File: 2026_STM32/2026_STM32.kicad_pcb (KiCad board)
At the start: 2 copper layers, 22 parts, among them J1 USB_B, J2 Conn_01x05_Pin, SW1 1825910-6, U1 SPX3819M5-L-3-3, U2 STM32C011F4P6, U3 KTD2026

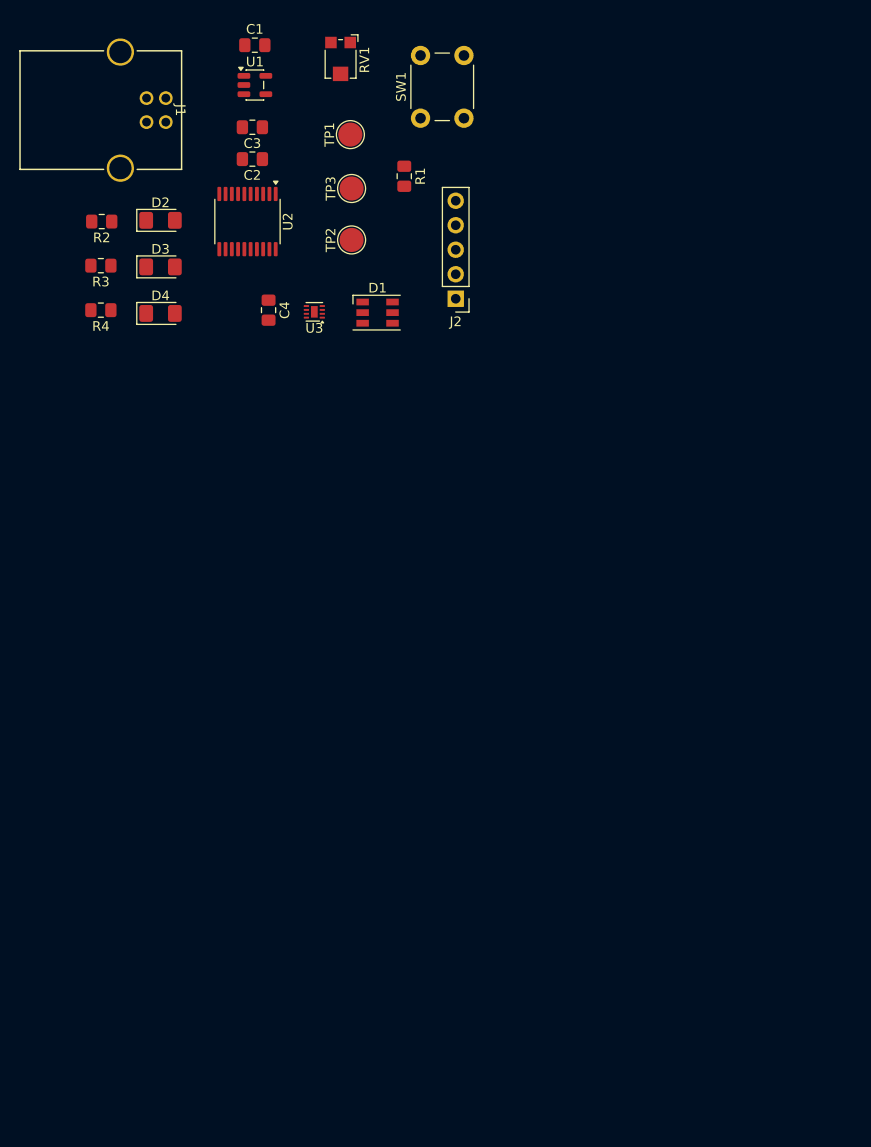
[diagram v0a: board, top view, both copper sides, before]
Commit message: stuff
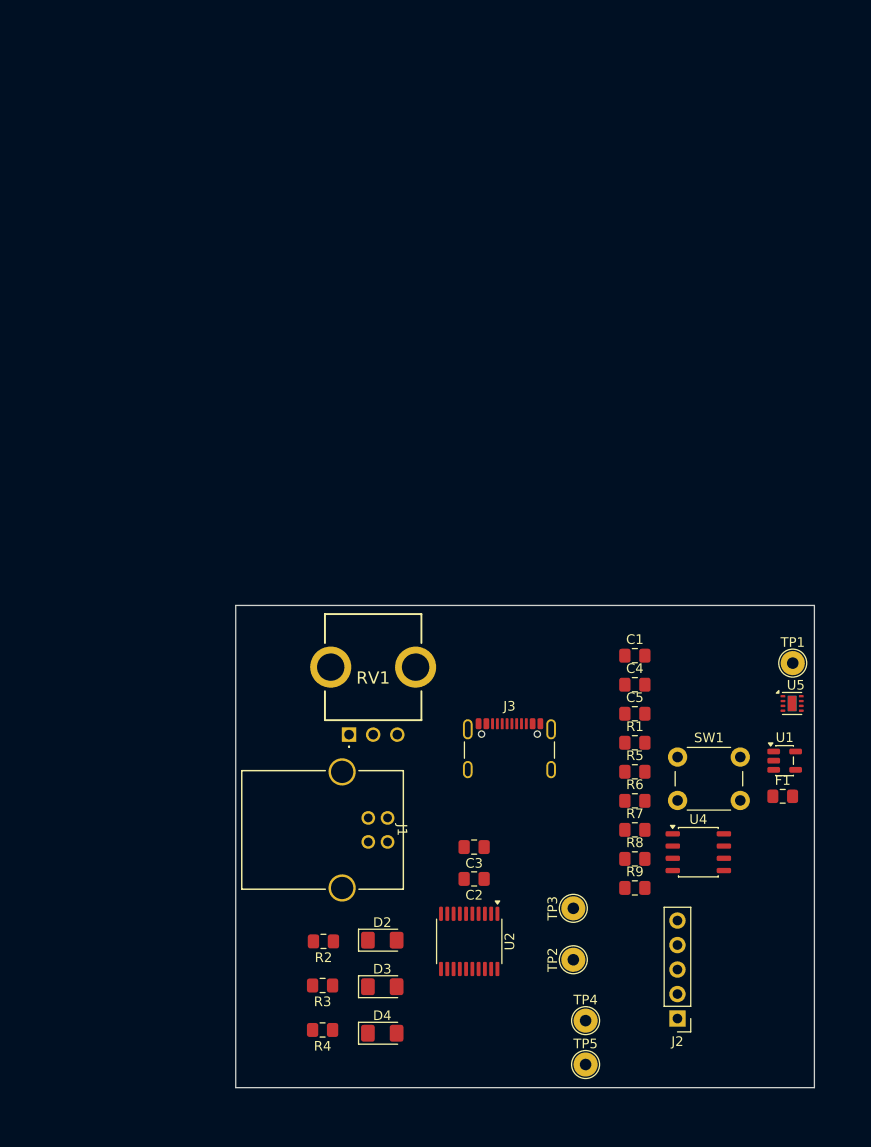
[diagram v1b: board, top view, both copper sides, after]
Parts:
- removed D1: CLX6F-FKC, LED_SMD:LED_RGB_PLCC-6
- removed U3: KTD2026, Package_DFN_QFN:DFN-8-1EP_1.5x1.5mm_P0.4mm_EP0.7x1.2mm
- added C5: 100nF, Capacitor_SMD:C_0805_2012Metric_Pad1.18x1.45mm_HandSolder, F.Cu at (141.4, 111.2)
- added F1: 0.5A, Fuse:Fuse_0805_2012Metric_Pad1.15x1.40mm_HandSolder, F.Cu at (156.7, 119.8)
- added J3: USB_C_Receptacle_USB2.0_16P, Connector_USB:USB_C_Receptacle_GCT_USB4105-xx-A_16P_TopMnt_Horizontal, F.Cu at (128.4, 115.9)
- added R5: 10kR, Capacitor_SMD:C_0805_2012Metric_Pad1.18x1.45mm_HandSolder, F.Cu at (141.4, 117.2)
- added R6: 10kR, Capacitor_SMD:C_0805_2012Metric_Pad1.18x1.45mm_HandSolder, F.Cu at (141.4, 120.3)
- added R7: 10kR, Capacitor_SMD:C_0805_2012Metric_Pad1.18x1.45mm_HandSolder, F.Cu at (141.4, 123.3)
- added R8: 5.1kR, Capacitor_SMD:C_0805_2012Metric_Pad1.18x1.45mm_HandSolder, F.Cu at (141.4, 126.3)
- added R9: 5.1kR, Capacitor_SMD:C_0805_2012Metric_Pad1.18x1.45mm_HandSolder, F.Cu at (141.4, 129.3)
- added TP4: TX, TestPoint:TestPoint_THTPad_D2.5mm_Drill1.2mm, F.Cu at (136.3, 143.1)
- added TP5: RX, TestPoint:TestPoint_THTPad_D2.5mm_Drill1.2mm, F.Cu at (136.3, 147.6)
- added U4: CH340N, Package_SO:JEITA_SOIC-8_3.9x4.9mm_P1.27mm, F.Cu at (148.0, 125.6)
- added U5: TMP1075DSG, Package_SON:WSON-8-1EP_2x2mm_P0.5mm_EP0.9x1.6mm_ThermalVias, F.Cu at (157.7, 110.2)
- C1: value 1.0uF -> 4.7uF
- C4: value 1.0uF -> 100nF
- R2: value 100R -> 330R
- RV1: footprint Potentiometer_SMD:Potentiometer_Bourns_TC33X_Vertical -> 2026 tutorial:PTV09A4015UB103
- TP1, TP2, TP3: footprint TestPoint:TestPoint_Pad_D2.5mm -> TestPoint:TestPoint_THTPad_D2.5mm_Drill1.2mm
- moved U1 89.0 mm to (156.9, 116.1)
- moved C3 78.1 mm to (124.7, 125.1)
- moved D4 78.1 mm to (115.2, 144.4)
- moved J1 78.1 mm to (115.7, 124.5)
- moved J2 78.1 mm to (145.8, 142.8)
- moved R3 78.1 mm to (109.0, 139.4)
- moved C2 78.1 mm to (124.7, 128.4)
- moved D2 78.1 mm to (115.2, 134.7)
- moved R2 78.1 mm to (109.1, 134.8)
- moved R4 78.1 mm to (109.0, 144.0)
- moved TP2 78.1 mm to (135.0, 136.7)
- moved TP3 78.1 mm to (135.0, 131.4)
- moved U2 78.1 mm to (124.2, 134.8)
- moved D3 78.1 mm to (115.2, 139.5)
- moved C1 74.6 mm to (141.4, 105.2), turned to 0 degrees
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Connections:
- D2 pad 2: /RED -> +3V3
- D3 pad 2: /GREEN -> +3V3
- D4 pad 2: /BLUE -> +3V3
- J1 pad 1: VBUS -> Net-(J1-VBUS)
- J1 pad 5: (no net) -> GND
- R1 pad 1: Net-(U2-PA1) -> Net-(U2-PA8)
- R2 pad 2: GND -> /RED
- R3 pad 2: GND -> /GREEN
- R4 pad 2: GND -> /BLUE
- RV1 pad 2: Net-(U2-PA0) -> Net-(U2-PA6)
- SW1 pad 1: Net-(U2-PA1) -> Net-(U2-PA8)
- TP1 pad 1: Net-(U2-PA0) -> Net-(U2-PA6)
- U2 pad 13: unconnected-(U2-PA6-Pad13) -> Net-(U2-PA6)
- U2 pad 15: unconnected-(U2-PA8-Pad15) -> Net-(U2-PA8)
- U2 pad 7: Net-(U2-PA0) -> /MCU_TX
- U2 pad 8: Net-(U2-PA1) -> /MCU_RX
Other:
- board outline added: 60 x 50 mm

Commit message: done
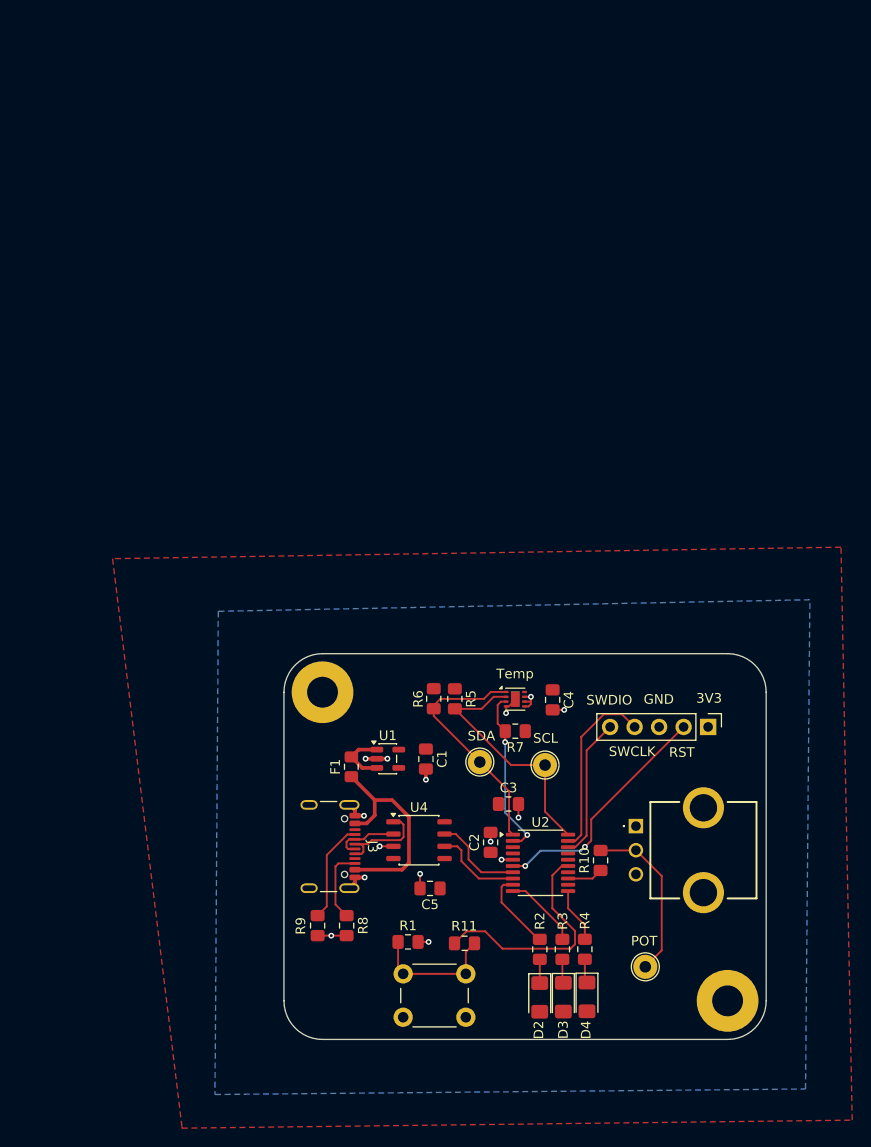
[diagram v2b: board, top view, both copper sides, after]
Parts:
- removed J1: USB_B, 2026 tutorial:CONN_USBB_12P04X10P62_AMP
- removed TP4: TX, TestPoint:TestPoint_THTPad_D2.5mm_Drill1.2mm
- removed TP5: RX, TestPoint:TestPoint_THTPad_D2.5mm_Drill1.2mm
- added H1: MountingHole_Pad, MountingHole:MountingHole_3.2mm_M3_Pad, F.Cu at (109.0, 109.0)
- added H2: MountingHole_Pad, MountingHole:MountingHole_3.2mm_M3_Pad, F.Cu at (151.0, 141.0)
- added R10: 330R, Capacitor_SMD:C_0805_2012Metric_Pad1.18x1.45mm_HandSolder, F.Cu at (137.8, 126.4)
- added R11: 330R, Capacitor_SMD:C_0805_2012Metric_Pad1.18x1.45mm_HandSolder, F.Cu at (123.7, 135.0)
- moved F1 44.8 mm to (112.0, 116.7), turned to 90 degrees
- moved U1 41.1 mm to (115.8, 115.9)
- moved SW1 36.3 mm to (117.4, 138.2)
- moved TP1 35.0 mm to (142.5, 137.5)
- moved R9 33.1 mm to (108.5, 133.2), turned to -90 degrees
- moved R1 31.3 mm to (117.9, 134.9)
- moved RV1 31.2 mm to (141.5, 122.9), turned to -90 degrees
- moved R8 30.7 mm to (111.5, 133.2), turned to -90 degrees
- moved J2 30.4 mm to (149.0, 112.6), turned to -90 degrees
- moved U4 29.0 mm to (119.0, 124.3)
- moved U5 28.7 mm to (129.0, 109.7)
- moved R4 28.5 mm to (136.2, 135.7), turned to 90 degrees
- moved C5 27.9 mm to (120.1, 129.3), turned to 180 degrees
- moved R3 25.1 mm to (133.9, 135.7), turned to 90 degrees
- moved C1 24.2 mm to (119.7, 115.9), turned to -90 degrees
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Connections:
- J2 pad 3: /SWCLK -> GND
- J2 pad 4: /SWDIO -> /SWCLK
- J2 pad 5: GND -> /SWDIO
- R1 pad 1: Net-(U2-PA8) -> Net-(R1-Pad1)
- R7 pad 2: /ALERT -> /Alert
- RV1 pad 2: Net-(U2-PA6) -> Net-(R10-Pad2)
- SW1 pad 1: Net-(U2-PA8) -> Net-(R1-Pad1)
- TP1 pad 1: Net-(U2-PA6) -> Net-(R10-Pad2)
- U2 pad 2: unconnected-(U2-PC14-Pad2) -> /Alert
- U5 pad 3: /ALERT -> /Alert
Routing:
- net /SCL: track 0.00 -> 25.8 mm
- net /~{RST}: track 0.00 -> 25.0 mm, vias 0 -> 2
- net /SDA: track 0.00 -> 24.9 mm
- net GND: track 0.00 -> 24.7 mm, vias 0 -> 15
- net Net-(U2-PA8): track 0.00 -> 24.1 mm
- net Net-(F1-Pad1): track 0.00 -> 22.4 mm
- net /SWCLK: track 0.00 -> 18.8 mm
- net Net-(R10-Pad2): track 0.00 -> 17.6 mm
- net /Alert: track 0.00 -> 17.5 mm, vias 0 -> 2
- net /SWDIO: track 0.00 -> 14.7 mm
- net Net-(R1-Pad1): track 0.00 -> 13.6 mm
- net Net-(J3-CC1): track 0.00 -> 10.5 mm
- net Net-(U4-UD+): track 0.00 -> 10.3 mm
- net /MCU_TX: track 0.00 -> 9.50 mm
- net /MCU_RX: track 0.00 -> 9.12 mm
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- added copper zone on F.Cu, net +3V3
- added copper zone on B.Cu, net GND
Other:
- board size 60 x 50 mm -> 50 x 40 mm
- board text added: "3V3"
- board text added: "GND"
- board text added: "POT"
- board text added: "RST"
- board text added: "SCL"
- board text added: "SDA"
- board text added: "SWCLK"
- board text added: "SWDIO"
- board text added: "Temp"
